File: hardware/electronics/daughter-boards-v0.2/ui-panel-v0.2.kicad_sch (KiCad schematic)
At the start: 9 parts

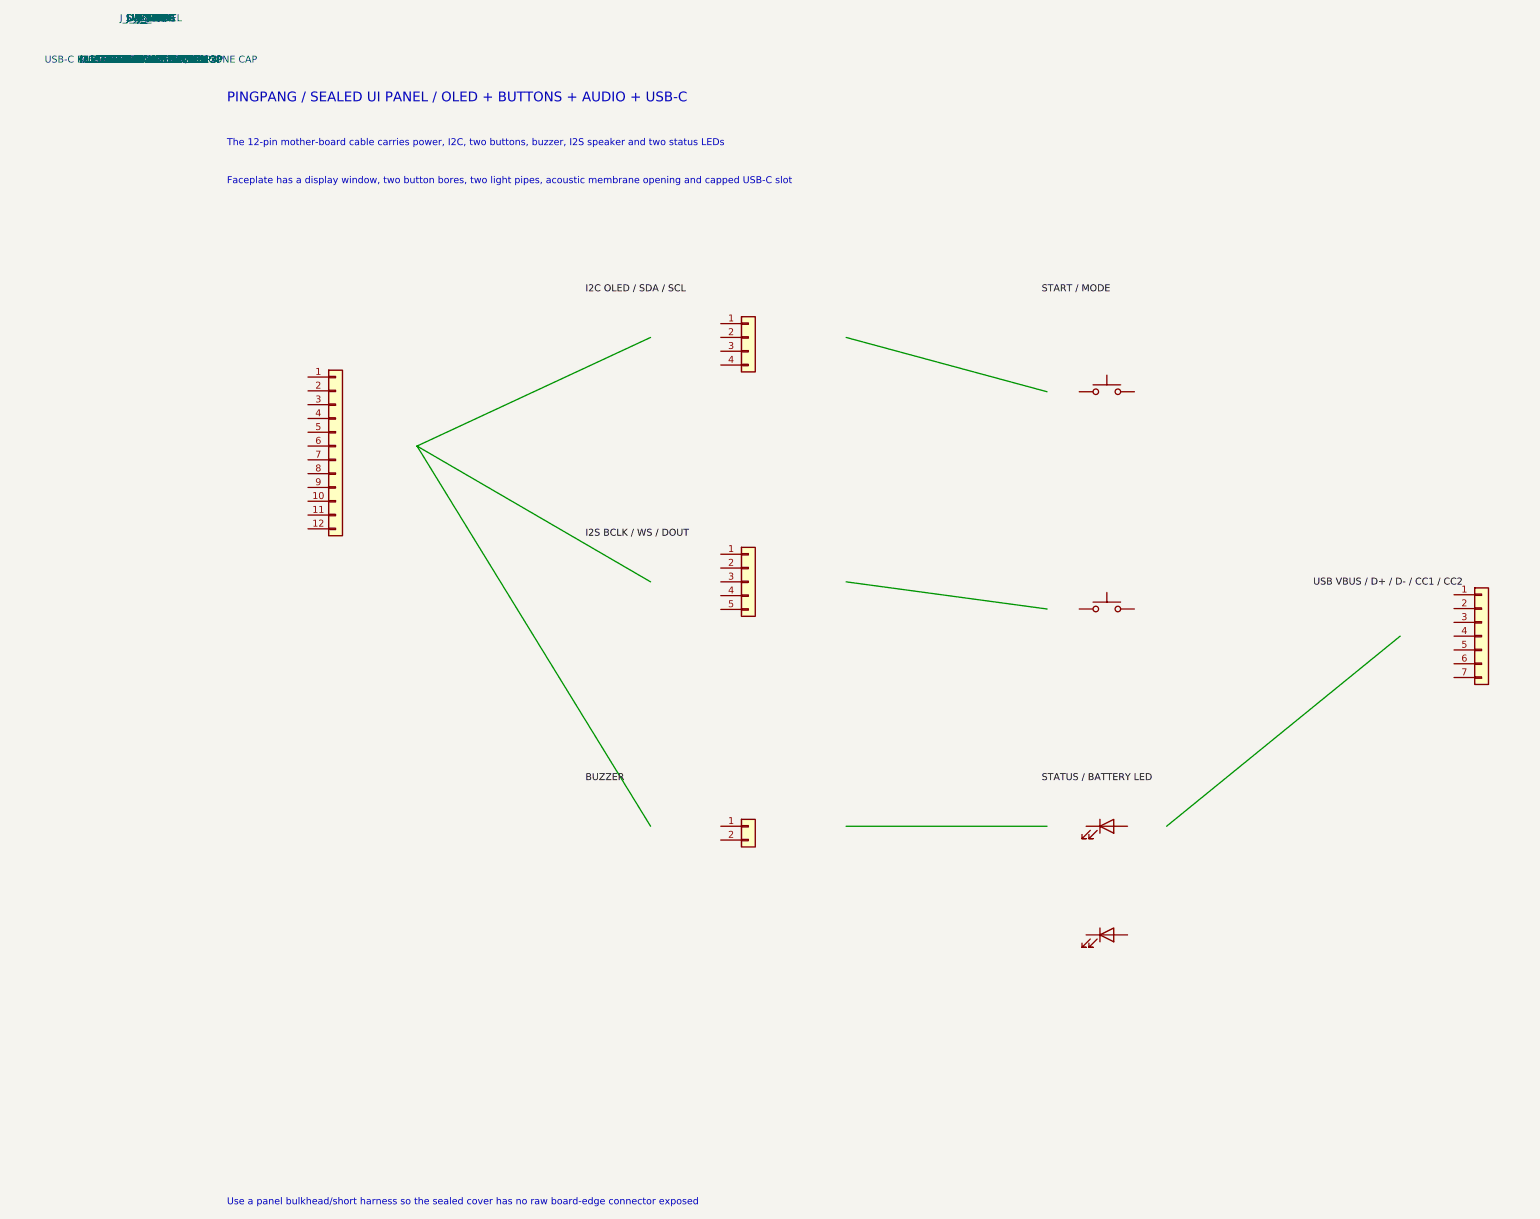
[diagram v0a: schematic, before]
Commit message: ✨ 完善面板接口对齐与打印预览
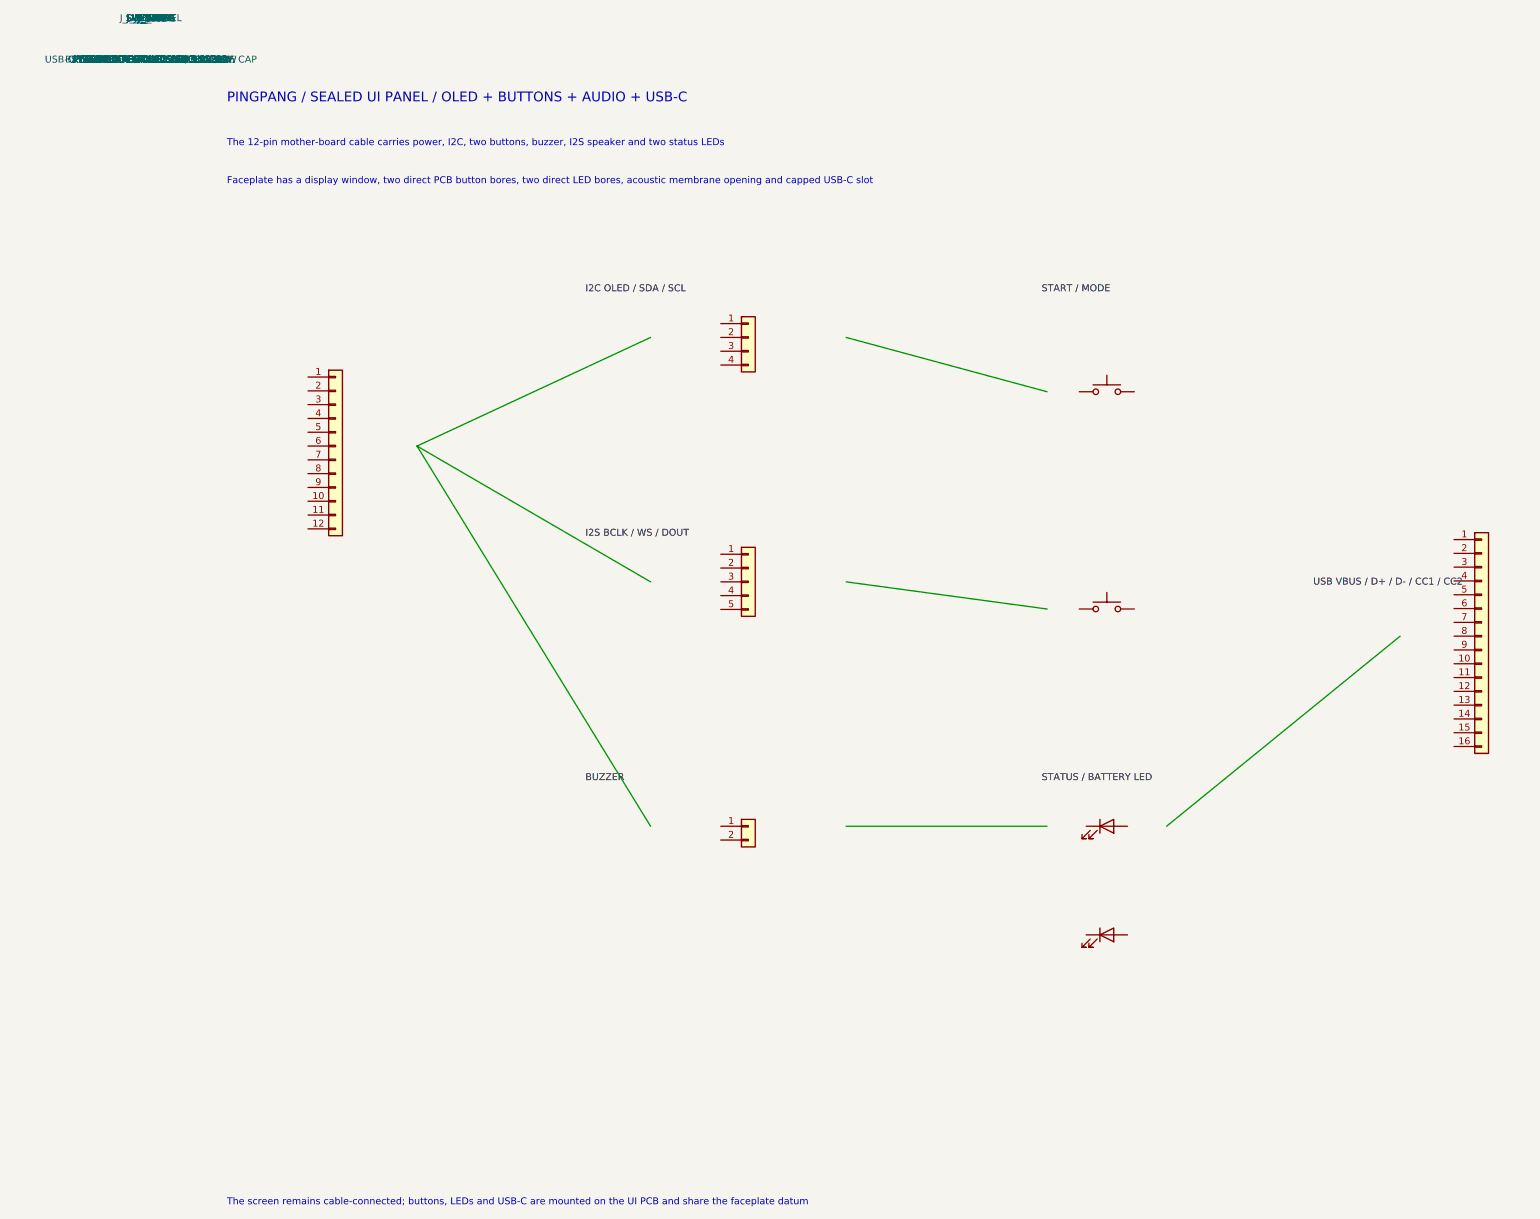
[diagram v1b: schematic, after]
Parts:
- removed J_USB_PANEL: USB-C BULKHEAD MX1.25 7P / SILICONE CAP, Connector_JST:JST_GH_SM07B-GHS-TB_1x07-1MP_P1.25mm_Horizontal, symbol Connector_Generic:Conn_01x07
- added J_USB_PANEL: USB-C VERTICAL 16P DIRECT / SILICONE CAP, Connector_USB:USB_C_Receptacle_G-Switch_GT-USB-7051x, symbol Connector_Generic:Conn_01x16
- D_BAT: value BATTERY LIGHT PIPE -> BATTERY DIRECT LED 0603 YELLOW
- D_STATUS: value STATUS LIGHT PIPE -> STATUS DIRECT LED 0603 GREEN
- J_OLED: value OLED I2C RESERVE MX1.25 4P -> OLED I2C FPC CABLE MX1.25 4P
- SW_MODE: value SEALED MODE BUTTON -> PCB DIRECT MODE SMD 3.9x3x2; footprint Button_Switch_SMD:SW_SPST_TL3301N160QG -> Button_Switch_SMD:SW_SPST_TS-1088-xR020
- SW_START: value SEALED START BUTTON -> PCB DIRECT START SMD 3.9x3x2; footprint Button_Switch_SMD:SW_SPST_TL3301N160QG -> Button_Switch_SMD:SW_SPST_TS-1088-xR020
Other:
- note added: "Faceplate has a display window, two direct PCB button bores, two direct LED bores, acoustic membrane opening and capped USB-C slot"
- note added: "The screen remains cable-connected; buttons, LEDs and USB-C are mounted on the UI PCB and share the faceplate datum"
- note removed: "Faceplate has a display window, two button bores, two light pipes, acoustic membrane opening and capped USB-C slot"
- note removed: "Use a panel bulkhead/short harness so the sealed cover has no raw board-edge connector exposed"
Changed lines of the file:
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@@
 		(effects (font (size 1.27 1.27)) (justify left bottom))
 	)
-	(text "Faceplate has a display window, two button bores, two light pipes, acoustic membrane opening and capped USB-C slot"
+	(text "Faceplate has a display window, two direct PCB button bores, two direct LED bores, acoustic membrane opening and capped USB-C slot"
 		(exclude_from_sim no)
 		(at 14 27 0)
 		(effects (font (size 1.27 1.27)) (justify left bottom))
 	)
-	(text "Use a panel bulkhead/short harness so the sealed cover has no raw board-edge connector exposed"
+	(text "The screen remains cable-connected; buttons, LEDs and USB-C are mounted on the UI PCB and share the faceplate datum"
 		(exclude_from_sim no)
 		(at 14 215 0)
@@
 		(instances
 			(project "ui-panel-v0.2"
-				(path "/d4aeef5e-0851-4b40-90a9-97642f63ddc4"
+				(path "/f68ee34d-60f0-4cb7-b441-7115130c09d0"
 					(reference "J_MOTHER")
 					(unit 1)
@@
 			)
 		)
-		(property "Value" "OLED I2C RESERVE MX1.25 4P"
+		(property "Value" "OLED I2C FPC CABLE MX1.25 4P"
 			(at 0 3.81 0)
 			(effects
@@
 		(instances
 			(project "ui-panel-v0.2"
-				(path "/d4aeef5e-0851-4b40-90a9-97642f63ddc4"
+				(path "/f68ee34d-60f0-4cb7-b441-7115130c09d0"
 					(reference "J_OLED")
 					(unit 1)
@@
 		(instances
 			(project "ui-panel-v0.2"
-				(path "/d4aeef5e-0851-4b40-90a9-97642f63ddc4"
+				(path "/f68ee34d-60f0-4cb7-b441-7115130c09d0"
 					(reference "J_SPK")
 					(unit 1)
@@
 		(instances
 			(project "ui-panel-v0.2"
-				(path "/d4aeef5e-0851-4b40-90a9-97642f63ddc4"
+				(path "/f68ee34d-60f0-4cb7-b441-7115130c09d0"
 					(reference "J_BUZ")
 					(unit 1)
@@
 			)
 		)
-		(property "Value" "SEALED START BUTTON"
-			(at 0 3.81 0)
-			(effects
-				(font
-					(size 1.27 1.27)
-				)
-			)
-		)
-		(property "Footprint" "Button_Switch_SMD:SW_SPST_TL3301N160QG"
-			(at 0 0 0)
-			(effects
-				(font
-					(size 1.27 1.27)
-				)
-				(hide yes)
-			)
-		)
-		(property "Datasheet" "~"
-			(at 0 0 0)
-			(effects
-				(font
-					(size 1.27 1.27)
-				)
-				(hide yes)
-			)
-		)
-		(property "Description" "Pingpang SmartGear connectorized control path"
-			(at 0 0 0)
-			(effects
-				(font
-					(size 1.27 1.27)
-				)
-				(hide yes)
-			)
-		)
-		(pin "1"
-		)
-		(pin "2"
-		)
-		(instances
-			(project "ui-panel-v0.2"
-				(path "/d4aeef5e-0851-4b40-90a9-97642f63ddc4"
+		(property "Value" "PCB DIRECT START SMD 3.9x3x2"
+			(at 0 3.81 0)
+			(effects
+				(font
+					(size 1.27 1.27)
+				)
+			)
+		)
+		(property "Footprint" "Button_Switch_SMD:SW_SPST_TS-1088-xR020"
+			(at 0 0 0)
+			(effects
+				(font
+					(size 1.27 1.27)
+				)
+				(hide yes)
+			)
+		)
+		(property "Datasheet" "~"
+			(at 0 0 0)
+			(effects
+				(font
+					(size 1.27 1.27)
+				)
+				(hide yes)
+			)
+		)
+		(property "Description" "Pingpang SmartGear connectorized control path"
+			(at 0 0 0)
+			(effects
+				(font
+					(size 1.27 1.27)
+				)
+				(hide yes)
+			)
+		)
+		(pin "1"
+		)
+		(pin "2"
+		)
+		(instances
+			(project "ui-panel-v0.2"
+				(path "/f68ee34d-60f0-4cb7-b441-7115130c09d0"
 					(reference "SW_START")
 					(unit 1)
@@
 			)
 		)
-		(property "Value" "SEALED MODE BUTTON"
-			(at 0 3.81 0)
-			(effects
-				(font
-					(size 1.27 1.27)
-				)
-			)
-		)
-		(property "Footprint" "Button_Switch_SMD:SW_SPST_TL3301N160QG"
-			(at 0 0 0)
-			(effects
-				(font
-					(size 1.27 1.27)
-				)
-				(hide yes)
-			)
-		)
-		(property "Datasheet" "~"
-			(at 0 0 0)
-			(effects
-				(font
-					(size 1.27 1.27)
-				)
-				(hide yes)
-			)
-		)
-		(property "Description" "Pingpang SmartGear connectorized control path"
-			(at 0 0 0)
-			(effects
-				(font
-					(size 1.27 1.27)
-				)
-				(hide yes)
-			)
-		)
-		(pin "1"
-		)
-		(pin "2"
-		)
-		(instances
-			(project "ui-panel-v0.2"
-				(path "/d4aeef5e-0851-4b40-90a9-97642f63ddc4"
+		(property "Value" "PCB DIRECT MODE SMD 3.9x3x2"
+			(at 0 3.81 0)
+			(effects
+				(font
+					(size 1.27 1.27)
+				)
+			)
+		)
+		(property "Footprint" "Button_Switch_SMD:SW_SPST_TS-1088-xR020"
+			(at 0 0 0)
+			(effects
+				(font
+					(size 1.27 1.27)
+				)
+				(hide yes)
+			)
+		)
+		(property "Datasheet" "~"
+			(at 0 0 0)
+			(effects
+				(font
+					(size 1.27 1.27)
+				)
+				(hide yes)
+			)
+		)
+		(property "Description" "Pingpang SmartGear connectorized control path"
+			(at 0 0 0)
+			(effects
+				(font
+					(size 1.27 1.27)
+				)
+				(hide yes)
+			)
+		)
+		(pin "1"
+		)
+		(pin "2"
+		)
+		(instances
+			(project "ui-panel-v0.2"
+				(path "/f68ee34d-60f0-4cb7-b441-7115130c09d0"
 					(reference "SW_MODE")
 					(unit 1)
@@
 			)
 		)
-		(property "Value" "STATUS LIGHT PIPE"
+		(property "Value" "STATUS DIRECT LED 0603 GREEN"
 			(at 0 3.81 0)
 			(effects
@@
 		(instances
 			(project "ui-panel-v0.2"
-				(path "/d4aeef5e-0851-4b40-90a9-97642f63ddc4"
+				(path "/f68ee34d-60f0-4cb7-b441-7115130c09d0"
 					(reference "D_STATUS")
 					(unit 1)
@@
 			)
 		)
-		(property "Value" "BATTERY LIGHT PIPE"
+		(property "Value" "BATTERY DIRECT LED 0603 YELLOW"
 			(at 0 3.81 0)
 			(effects
@@
 		(instances
 			(project "ui-panel-v0.2"
-				(path "/d4aeef5e-0851-4b40-90a9-97642f63ddc4"
+				(path "/f68ee34d-60f0-4cb7-b441-7115130c09d0"
 					(reference "D_BAT")
 					(unit 1)
@@
 	)
 	(symbol
-		(lib_id "Connector_Generic:Conn_01x07")
+		(lib_id "Connector_Generic:Conn_01x16")
 		(at 245 110 0)
 		(unit 1)
@@
 			)
 		)
-		(property "Value" "USB-C BULKHEAD MX1.25 7P / SILICONE CAP"
-			(at 0 3.81 0)
-			(effects
-				(font
-					(size 1.27 1.27)
-				)
-			)
-		)
-		(property "Footprint" "Connector_JST:JST_GH_SM07B-GHS-TB_1x07-1MP_P1.25mm_Horizontal"
+		(property "Value" "USB-C VERTICAL 16P DIRECT / SILICONE CAP"
+			(at 0 3.81 0)
+			(effects
+				(font
+					(size 1.27 1.27)
+				)
+			)
+		)
+		(property "Footprint" "Connector_USB:USB_C_Receptacle_G-Switch_GT-USB-7051x"
 			(at 0 0 0)
 			(effects
@@
 		(pin "7"
 		)
-		(instances
-			(project "ui-panel-v0.2"
-				(path "/d4aeef5e-0851-4b40-90a9-97642f63ddc4"
+		(pin "8"
+		)
+		(pin "9"
+		)
+		(pin "10"
+		)
+		(pin "11"
+		)
+		(pin "12"
+		)
+		(pin "13"
+		)
+		(pin "14"
+		)
+		(pin "15"
+		)
+		(pin "16"
+		)
+		(instances
+			(project "ui-panel-v0.2"
+				(path "/f68ee34d-60f0-4cb7-b441-7115130c09d0"
 					(reference "J_USB_PANEL")
 					(unit 1)
